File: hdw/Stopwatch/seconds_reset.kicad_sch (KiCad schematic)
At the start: 21 parts, among them U1301 74LVC1G97, U1302 74LVC1G97, U1303 74LVC1G97, U1304 74LVC1G97, U1305 74LVC1G97, U1306 74LVC1G97, U1307 74LVC1G97

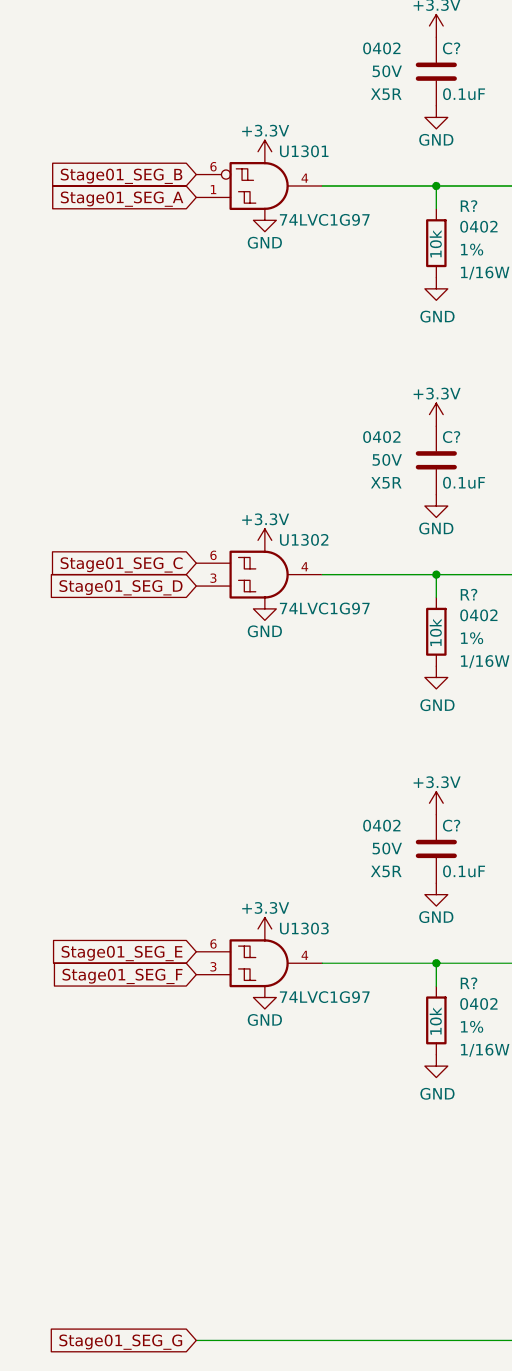
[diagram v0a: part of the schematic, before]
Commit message: lots and lots of routing
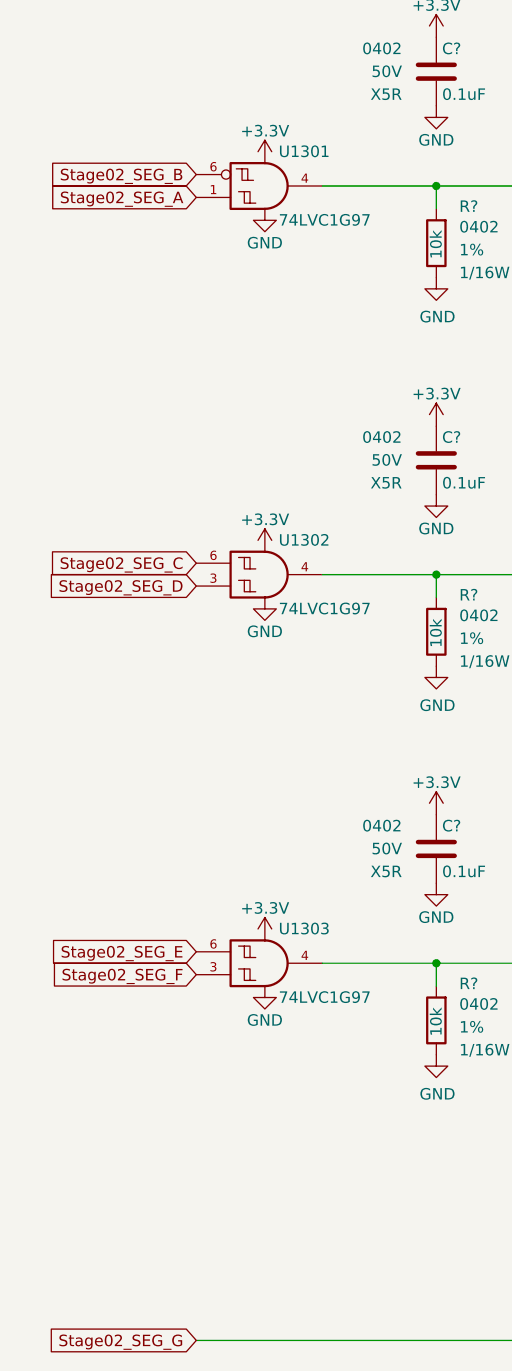
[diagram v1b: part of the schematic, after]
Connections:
- net +3V3 is gone; now on net +3.3V: C?.1, C?.1, C?.1, C?.1, C?.1, C?.1, C?.1
- net Stage01_SEG_A renamed Stage02_SEG_A
- net Stage01_SEG_B renamed Stage02_SEG_B
- net Stage01_SEG_C renamed Stage02_SEG_C
- net Stage01_SEG_D renamed Stage02_SEG_D
- net Stage01_SEG_E renamed Stage02_SEG_E
- net Stage01_SEG_F renamed Stage02_SEG_F
- net Stage01_SEG_G renamed Stage02_SEG_G
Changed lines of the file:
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@@
     (stroke (width 0) (type default))
   )
-  (global_label "Stage01_SEG_E" (shape input) (at 43.18 124.46 180) (fields_autoplaced)
+  (global_label "Stage02_SEG_E" (shape input) (at 43.18 124.46 180) (fields_autoplaced)
     (effects (font (size 1.27 1.27)) (justify right))
     (property "Intersheetrefs" "${INTERSHEET_REFS}" (at 26.4749 124.46 0)
@@
     )
   )
-  (global_label "Stage01_SEG_A" (shape input) (at 43.18 40.64 180) (fields_autoplaced)
+  (global_label "Stage02_SEG_A" (shape input) (at 43.18 40.64 180) (fields_autoplaced)
     (effects (font (size 1.27 1.27)) (justify right))
     (property "Intersheetrefs" "${INTERSHEET_REFS}" (at 26.5353 40.64 0)
@@
     )
   )
-  (global_label "Stage01_SEG_D" (shape input) (at 43.18 83.82 180) (fields_autoplaced)
+  (global_label "Stage02_SEG_D" (shape input) (at 43.18 83.82 180) (fields_autoplaced)
     (effects (font (size 1.27 1.27)) (justify right))
     (property "Intersheetrefs" "${INTERSHEET_REFS}" (at 26.3539 83.82 0)
@@
     )
   )
-  (global_label "Stage01_SEG_F" (shape input) (at 43.18 127 180) (fields_autoplaced)
+  (global_label "Stage02_SEG_F" (shape input) (at 43.18 127 180) (fields_autoplaced)
     (effects (font (size 1.27 1.27)) (justify right))
     (property "Intersheetrefs" "${INTERSHEET_REFS}" (at 26.5353 127 0)
@@
     )
   )
-  (global_label "Stage01_SEG_G" (shape input) (at 43.18 167.64 180) (fields_autoplaced)
+  (global_label "Stage02_SEG_G" (shape input) (at 43.18 167.64 180) (fields_autoplaced)
     (effects (font (size 1.27 1.27)) (justify right))
     (property "Intersheetrefs" "${INTERSHEET_REFS}" (at 26.3539 167.64 0)
@@
     )
   )
-  (global_label "Stage01_SEG_C" (shape input) (at 43.18 81.28 180) (fields_autoplaced)
+  (global_label "Stage02_SEG_C" (shape input) (at 43.18 81.28 180) (fields_autoplaced)
     (effects (font (size 1.27 1.27)) (justify right))
     (property "Intersheetrefs" "${INTERSHEET_REFS}" (at 26.3539 81.28 0)
@@
     )
   )
-  (global_label "Stage01_SEG_B" (shape input) (at 43.18 38.1 180) (fields_autoplaced)
+  (global_label "Stage02_SEG_B" (shape input) (at 43.18 38.1 180) (fields_autoplaced)
     (effects (font (size 1.27 1.27)) (justify right))
     (property "Intersheetrefs" "${INTERSHEET_REFS}" (at 26.3539 38.1 0)
@@
     )
   )
-  (symbol (lib_id "Incrementor-rescue:+3.3V-power") (at 223.52 22.86 0) (unit 1)
+  (symbol (lib_id "power:+3.3V") (at 223.52 22.86 0) (unit 1)
     (in_bom yes) (on_board yes) (dnp no)
     (property "Reference" "#PWR?" (at 223.52 26.67 0)
@@
     )
   )
-  (symbol (lib_id "Incrementor-rescue:+3.3V-power") (at 69.85 66.04 0) (unit 1)
+  (symbol (lib_id "power:+3.3V") (at 69.85 66.04 0) (unit 1)
     (in_bom yes) (on_board yes) (dnp no)
     (property "Reference" "#PWR?" (at 69.85 69.85 0)
@@
     )
   )
-  (symbol (lib_id "Incrementor-rescue:+3.3V-power") (at 69.85 109.22 0) (unit 1)
+  (symbol (lib_id "power:+3.3V") (at 69.85 109.22 0) (unit 1)
     (in_bom yes) (on_board yes) (dnp no)
     (property "Reference" "#PWR?" (at 69.85 113.03 0)
@@
     )
   )
-  (symbol (lib_id "Incrementor-rescue:+3.3V-power") (at 172.72 22.86 0) (unit 1)
+  (symbol (lib_id "power:+3.3V") (at 172.72 22.86 0) (unit 1)
     (in_bom yes) (on_board yes) (dnp no)
     (property "Reference" "#PWR?" (at 172.72 26.67 0)
@@
     )
   )
-  (symbol (lib_id "Incrementor-rescue:+3.3V-power") (at 120.65 22.86 0) (unit 1)
+  (symbol (lib_id "power:+3.3V") (at 120.65 22.86 0) (unit 1)
     (in_bom yes) (on_board yes) (dnp no)
     (property "Reference" "#PWR?" (at 120.65 26.67 0)
@@
     )
   )
-  (symbol (lib_id "Incrementor-rescue:+3.3V-power") (at 120.65 109.22 0) (unit 1)
+  (symbol (lib_id "power:+3.3V") (at 120.65 109.22 0) (unit 1)
     (in_bom yes) (on_board yes) (dnp no)
     (property "Reference" "#PWR?" (at 120.65 113.03 0)
@@
     )
   )
-  (symbol (lib_id "Incrementor-rescue:+3.3V-power") (at 69.85 22.86 0) (unit 1)
+  (symbol (lib_id "power:+3.3V") (at 69.85 22.86 0) (unit 1)
     (in_bom yes) (on_board yes) (dnp no)
     (property "Reference" "#PWR?" (at 69.85 26.67 0)

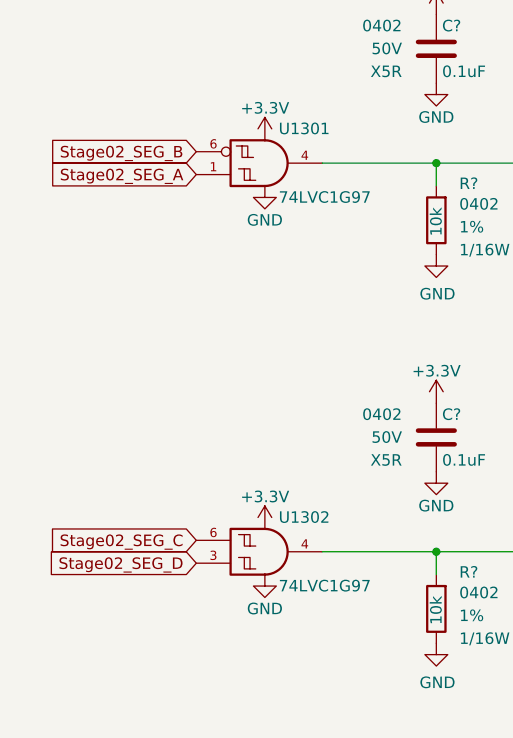
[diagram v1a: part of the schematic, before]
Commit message: got no unconnects to 0
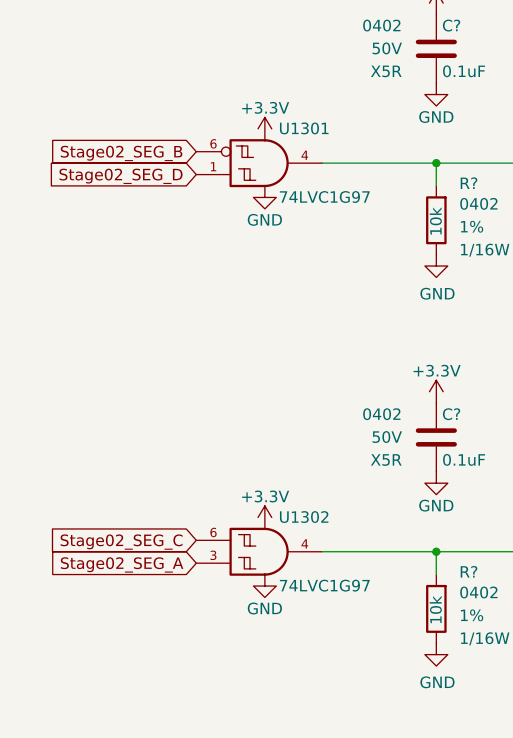
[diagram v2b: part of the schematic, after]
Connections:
- net Stage02_SEG_A: now also U1302.3; no longer U1301.1
- net Stage02_SEG_D: now also U1301.1; no longer U1302.3
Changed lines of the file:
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@@
     )
   )
-  (global_label "Stage02_SEG_A" (shape input) (at 43.18 40.64 180) (fields_autoplaced)
+  (global_label "Stage02_SEG_A" (shape input) (at 43.18 83.82 180) (fields_autoplaced)
     (effects (font (size 1.27 1.27)) (justify right))
-    (property "Intersheetrefs" "${INTERSHEET_REFS}" (at 26.5353 40.64 0)
+    (property "Intersheetrefs" "${INTERSHEET_REFS}" (at 26.5353 83.82 0)
       (effects (font (size 1.27 1.27)) (justify right) hide)
     )
   )
-  (global_label "Stage02_SEG_D" (shape input) (at 43.18 83.82 180) (fields_autoplaced)
+  (global_label "Stage02_SEG_D" (shape input) (at 43.18 40.64 180) (fields_autoplaced)
     (effects (font (size 1.27 1.27)) (justify right))
-    (property "Intersheetrefs" "${INTERSHEET_REFS}" (at 26.3539 83.82 0)
+    (property "Intersheetrefs" "${INTERSHEET_REFS}" (at 26.3539 40.64 0)
       (effects (font (size 1.27 1.27)) (justify right) hide)
     )
